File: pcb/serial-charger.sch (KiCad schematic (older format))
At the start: 24 parts, among them IC1 CH340G, IC2 TP4056, J1 jumper, J2 jumper, J3 jumper, J4 jumper, P1 CONN_01X01, P2 USB_OTG, P3 CONN_01X05, P4 CONN_01X01, U1 XC6206, x1 xtal_osc

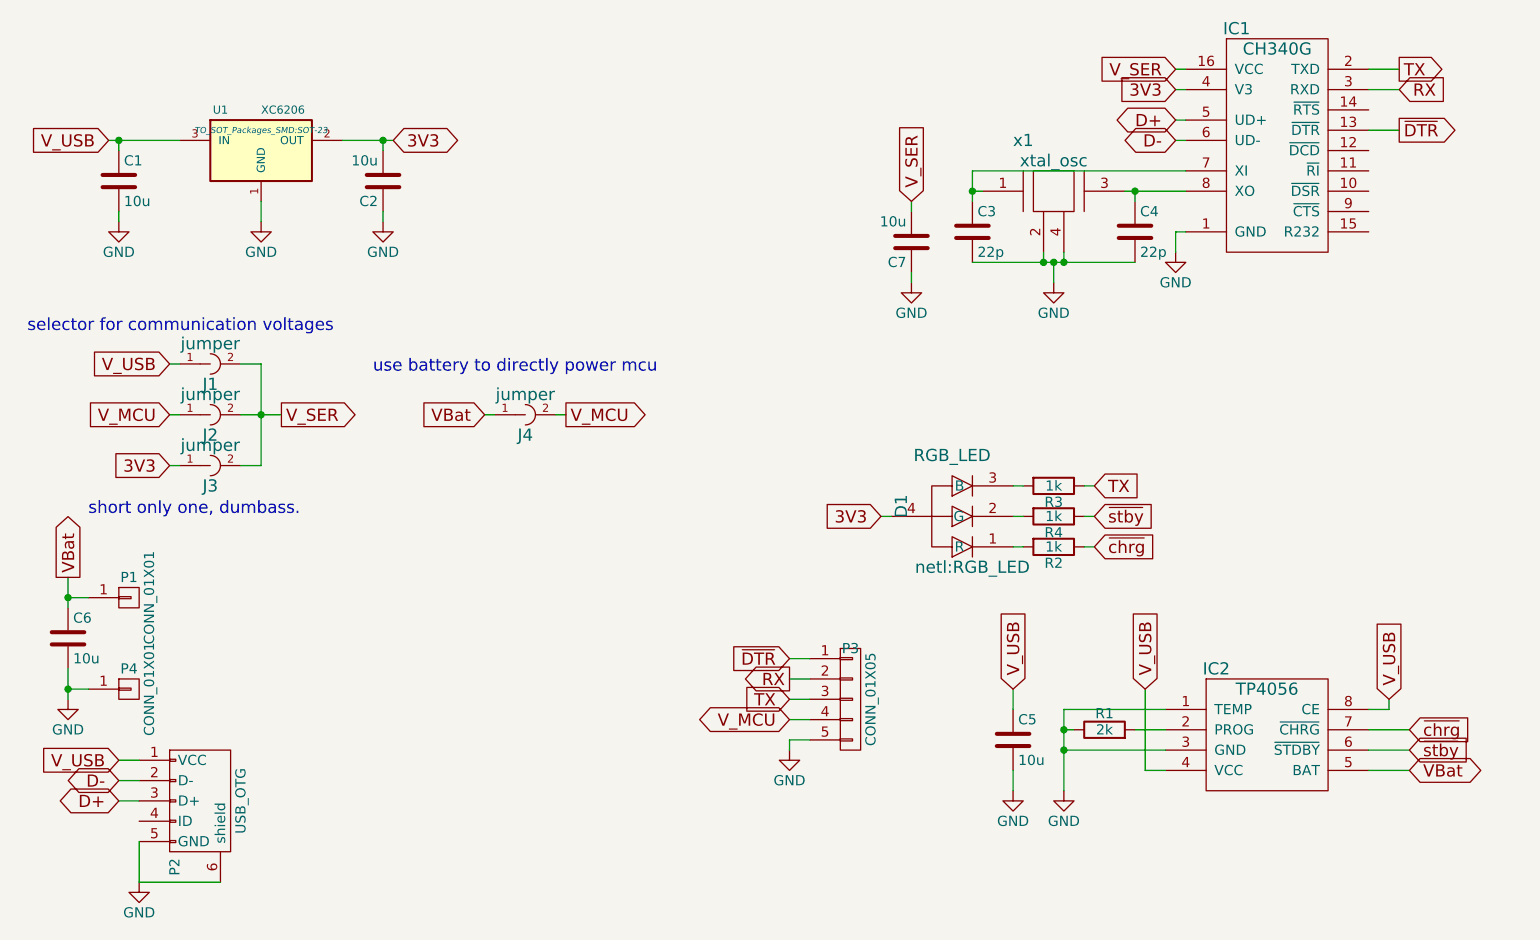
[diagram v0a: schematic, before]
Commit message: changed charger
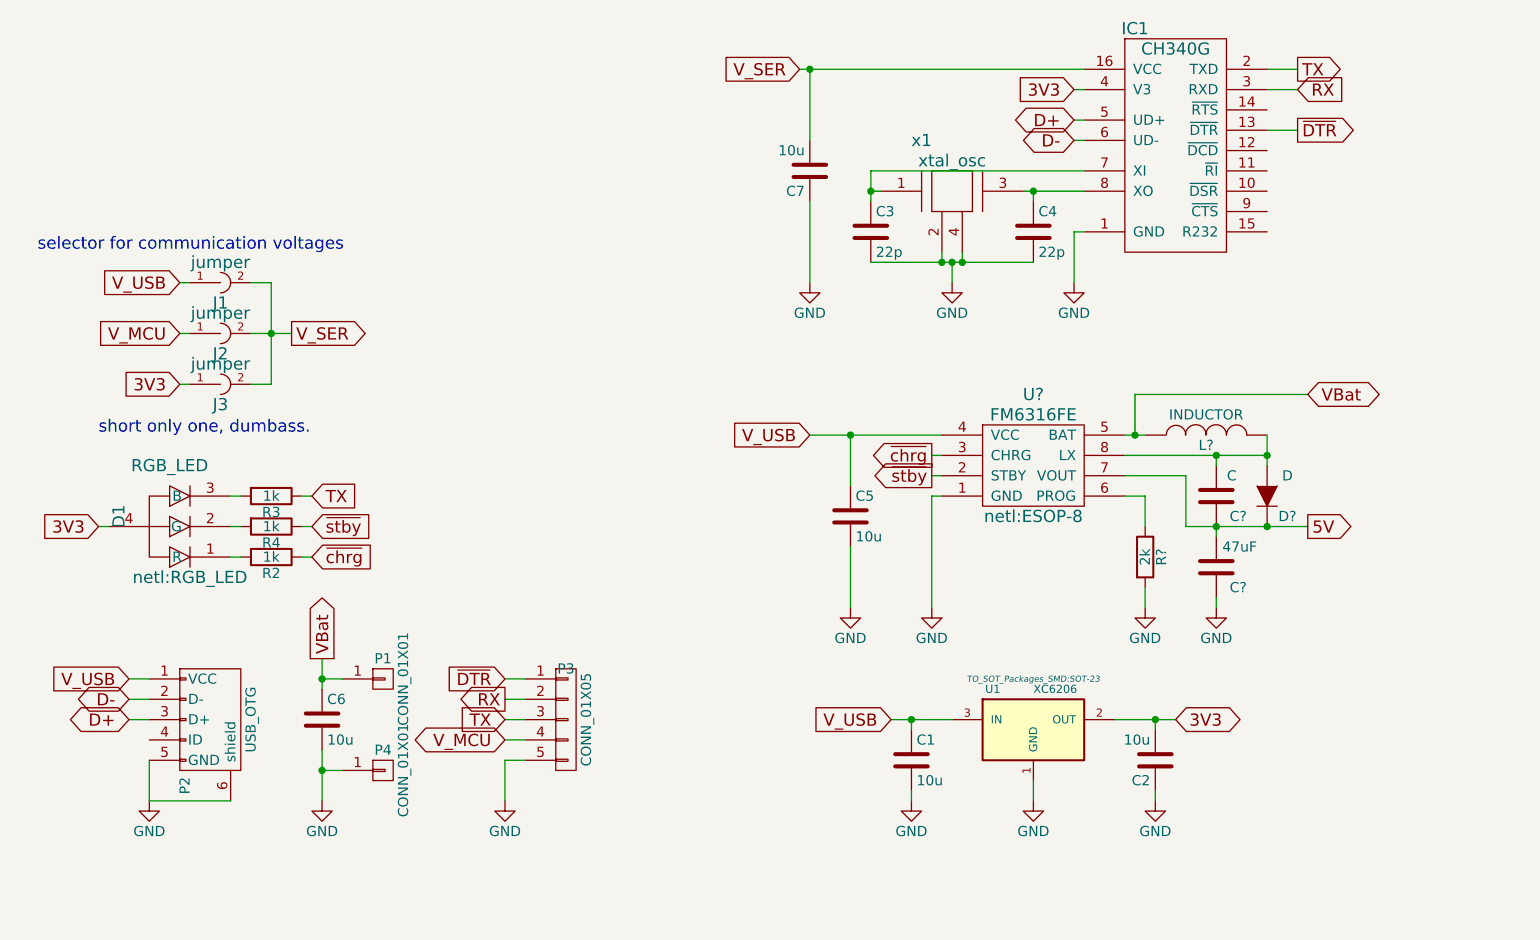
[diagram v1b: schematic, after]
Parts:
- removed IC2: TP4056, SMD_Packages:SOIC-8-N, symbol TP4056
- removed J4: jumper, netl:Jumper, symbol jumper
- removed R1: 2k, netl:SMD_0603, symbol R
- added C?: C, symbol C
- added C?: 47uF, symbol C
- added D?: D, symbol D
- added L?: INDUCTOR, symbol INDUCTOR
- added R?: 2k, netl:SMD_0603, symbol R
- added U?: FM6316FE, netl:ESOP-8, symbol FM6316FE
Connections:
- net GND: now also C?.1, R?.2, U?.1 (GND)
- net VBat: now also L?.1, U?.5 (BAT)
- net V_USB: now also U?.4 (VCC)
- net ~chrg: now also U?.3 (CHRG)
- net ~stby: now also U?.2 (STBY)
- new net: R?.1, U?.6 (PROG)
- new net: C?.2, D?.2 (A), L?.2, U?.8 (LX)
- new net 5V: C?.1, C?.2, D?.1 (K), U?.7 (VOUT)
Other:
- note removed: "use battery to directly power mcu"
- moved on the sheet: C1, C2, C3, C4, C5, C6, C7, D1, IC1, J1, J2, J3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
